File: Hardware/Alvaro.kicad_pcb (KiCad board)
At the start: 2 copper layers, 17.8 x 33 mm, 27 parts, among them J2 01x02, J3 01x12, J4 01x12, J5 01x05, P1 USB_C_Receptacle_USB2.0, U1 ATmega32U4, X1 16MHz

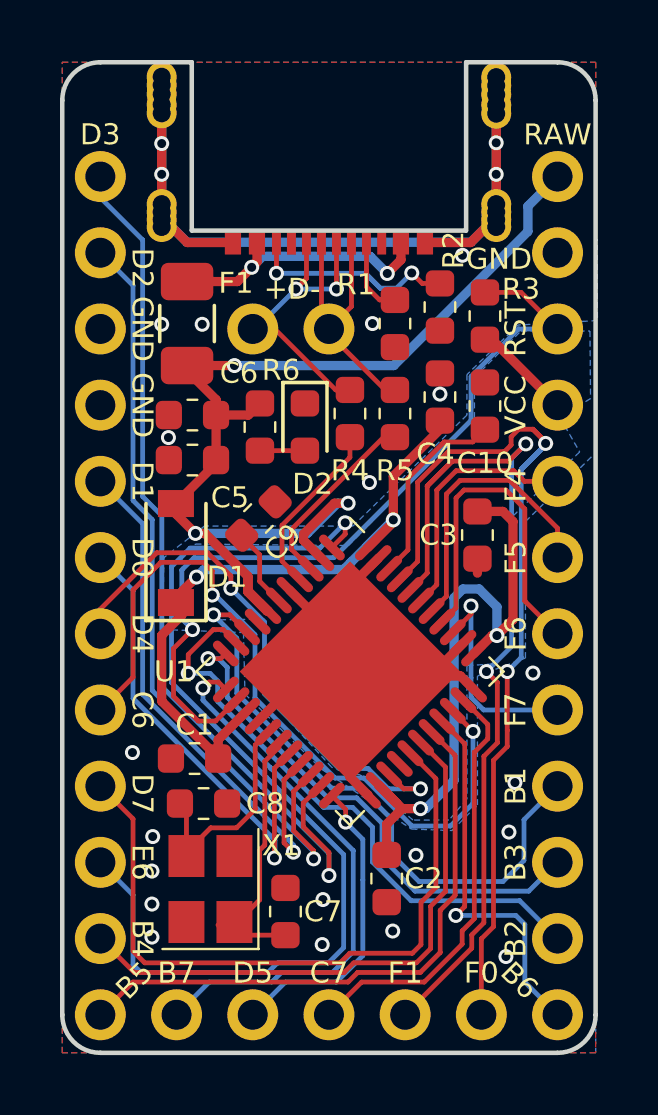
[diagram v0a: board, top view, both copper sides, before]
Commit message: Added THT pad under the 32u4.
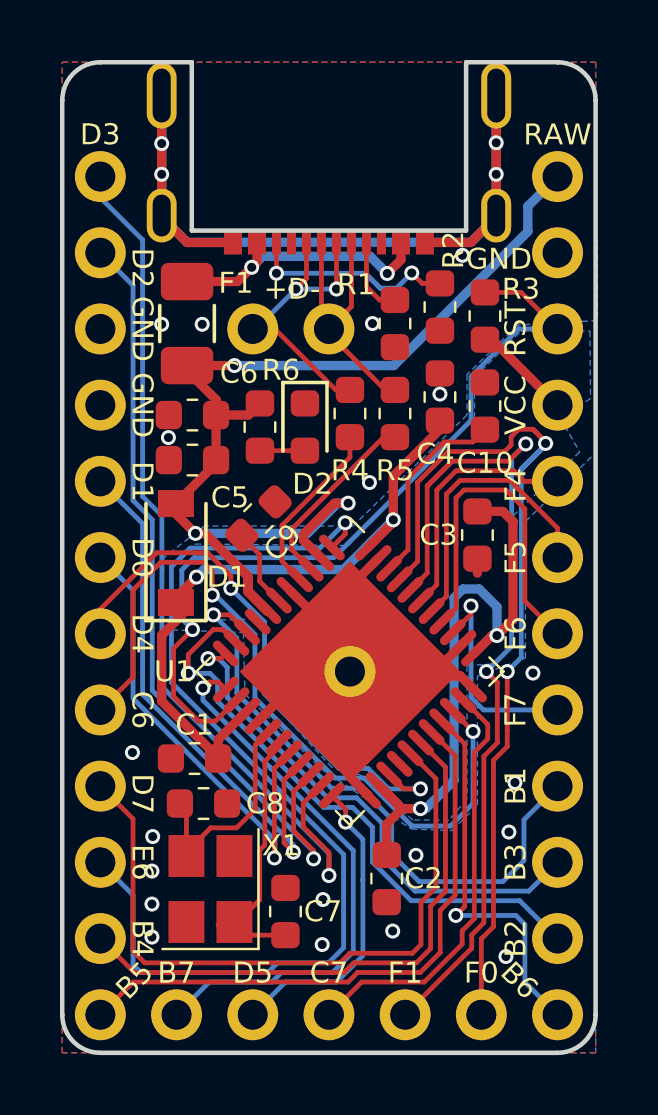
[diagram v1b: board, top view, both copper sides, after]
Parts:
- P1: footprint Alvaro:USB-C_C168688 -> Alvaro:USB-C-C168688
- R6: value 10k -> 1k

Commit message: Revert "Added THT pad under the 32u4."
This reverts commit 5261bc7efe342fde01f2eec8e41c6f0668064f92.
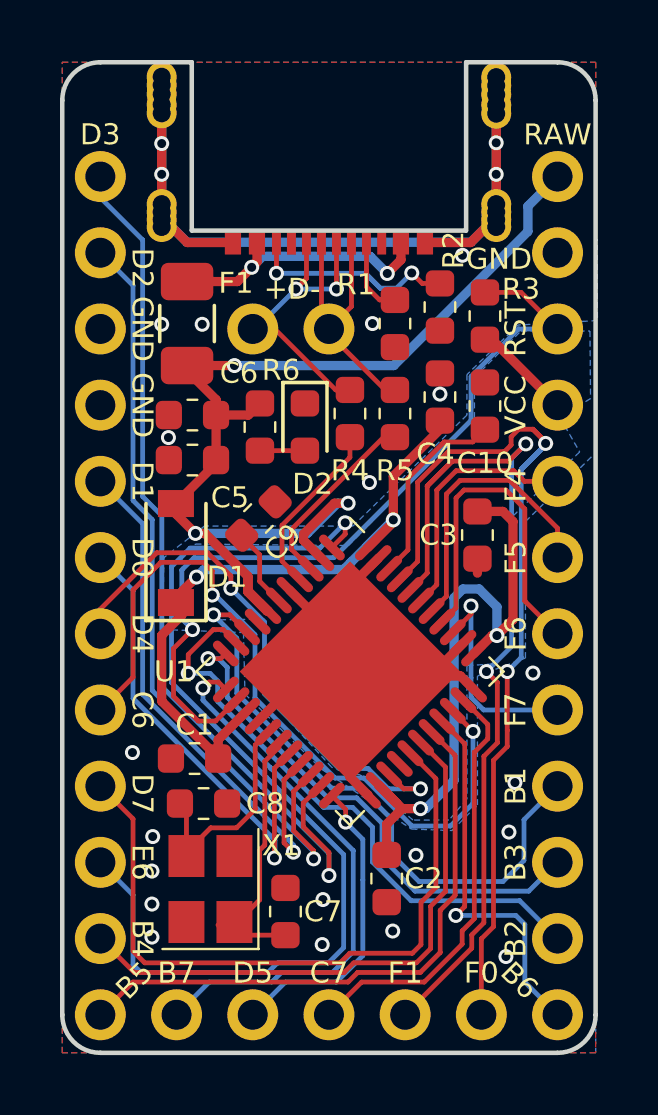
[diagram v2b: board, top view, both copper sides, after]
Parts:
- P1: footprint Alvaro:USB-C-C168688 -> Alvaro:USB-C_C168688
- R6: value 1k -> 10k
